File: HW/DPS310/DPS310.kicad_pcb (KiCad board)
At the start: 2 copper layers, 32.2 x 27.4 mm, 8 parts, among them J1 Screw_Terminal_01x06, U1 DPS310

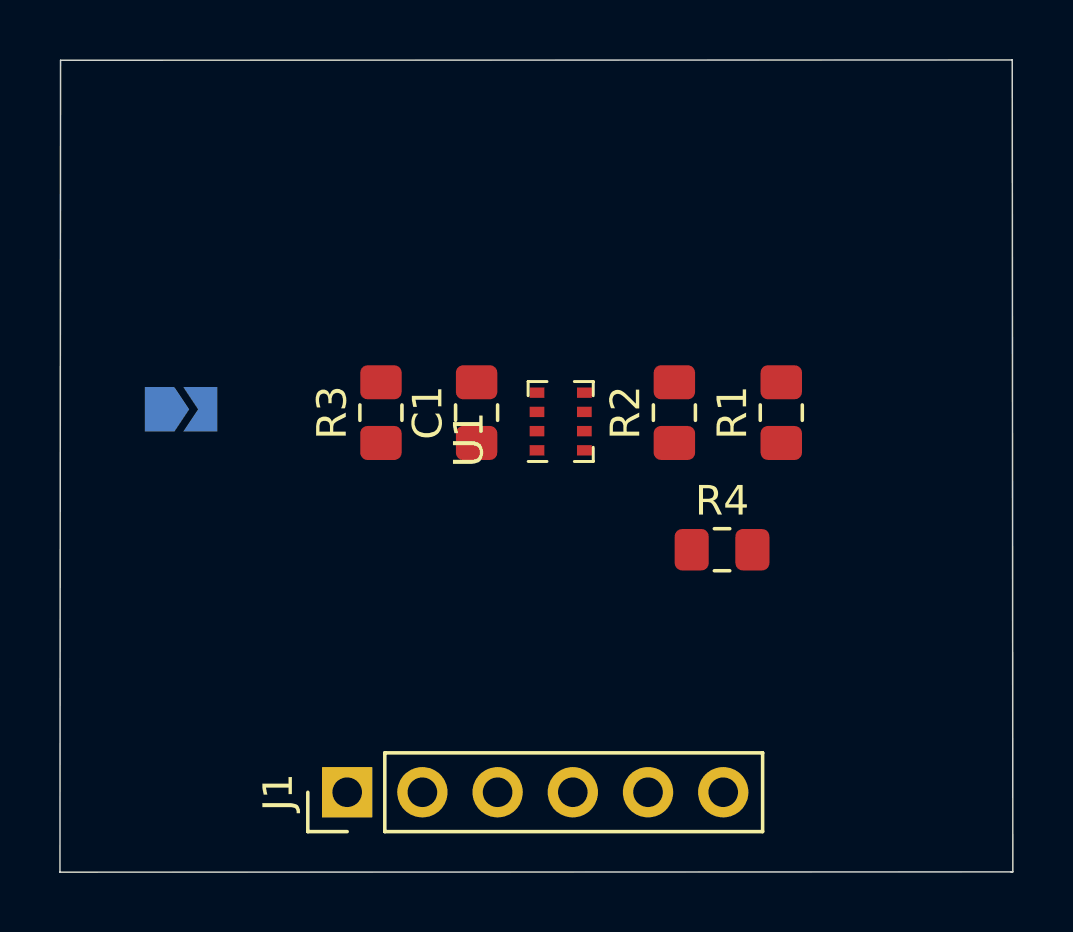
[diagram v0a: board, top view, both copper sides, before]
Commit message: Last revision of PCB
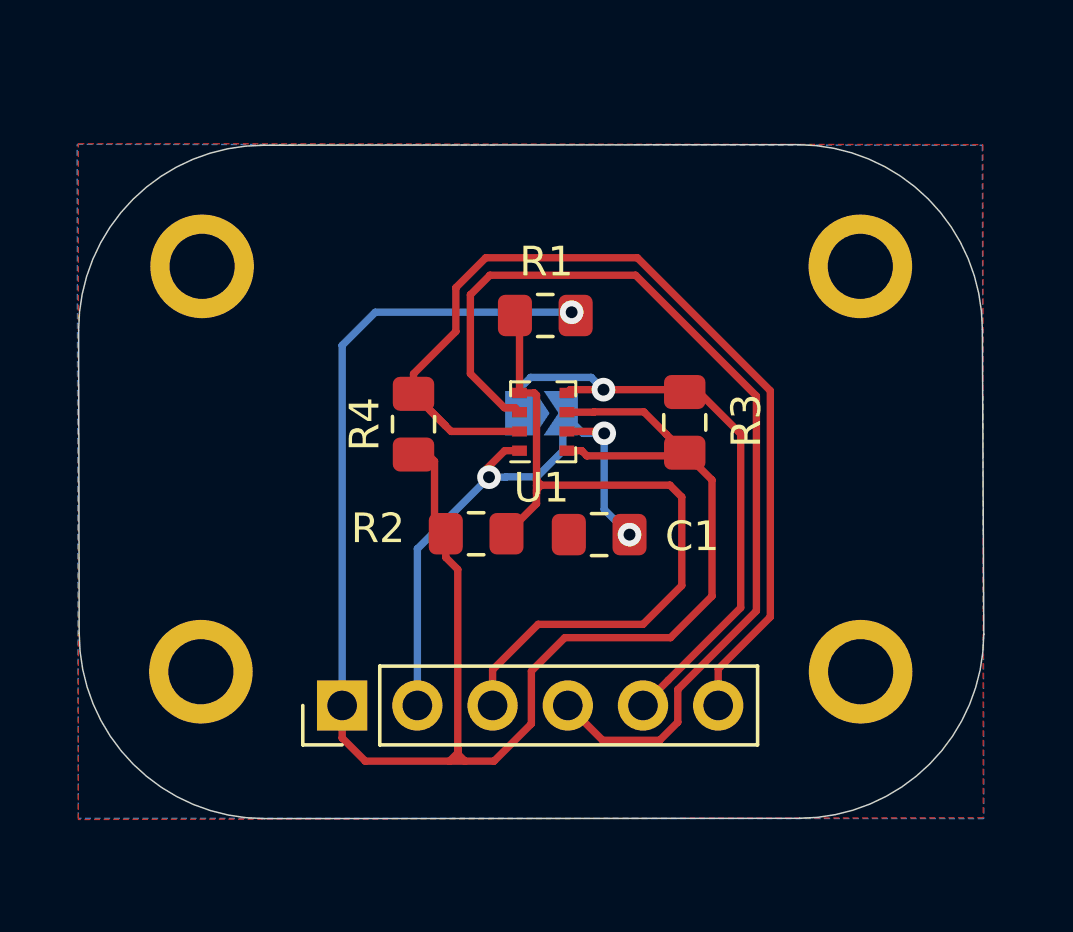
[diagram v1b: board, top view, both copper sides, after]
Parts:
- added REF**: MountingHole_2.2mm_M2_ISO7380_Pad, MountingHole:MountingHole_2.2mm_M2_ISO7380_Pad, F.Cu at (136.9, 78.5)
- added REF**: MountingHole_2.2mm_M2_ISO7380_Pad, MountingHole:MountingHole_2.2mm_M2_ISO7380_Pad, F.Cu at (114.7, 78.5)
- added REF**: MountingHole_2.2mm_M2_ISO7380_Pad, MountingHole:MountingHole_2.2mm_M2_ISO7380_Pad, F.Cu at (114.6, 92.2)
- added REF**: MountingHole_2.2mm_M2_ISO7380_Pad, MountingHole:MountingHole_2.2mm_M2_ISO7380_Pad, F.Cu at (136.9, 92.2)
- moved JP1 12.2 mm to (126.1, 83.4)
- moved R4 11.2 mm to (121.8, 83.8), turned to 90 degrees
- moved R3 10.3 mm to (131.0, 83.7)
- moved R1 8.62 mm to (126.2, 80.1), turned to 180 degrees
- moved R2 7.85 mm to (123.9, 87.5), turned to 0 degrees
- moved C1 5.84 mm to (128.1, 87.5), turned to 0 degrees
- moved J1 2.93 mm to (119.4, 93.3)
- moved U1 0.59 mm to (126.2, 83.7)
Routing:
- net VCC: track 0.00 -> 63.4 mm, vias 0 -> 1
- net /CS: track 0.00 -> 33.3 mm
- net /SDI_SDA: track 0.00 -> 33.1 mm
- net /SCL_SCK: track 0.00 -> 25.8 mm
- net GND: track 0.00 -> 21.3 mm, vias 0 -> 3
- net /SDO_ADR: track 0.00 -> 21.1 mm, vias 0 -> 1
- added copper zone on B.Cu, net (none)
- added copper zone on F.Cu, net GND
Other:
- board size 32.2 x 27.4 mm -> 30.6 x 22.8 mm
